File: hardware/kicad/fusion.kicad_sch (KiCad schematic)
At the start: 7 parts, among them J1 Battery, U1 MCP1603

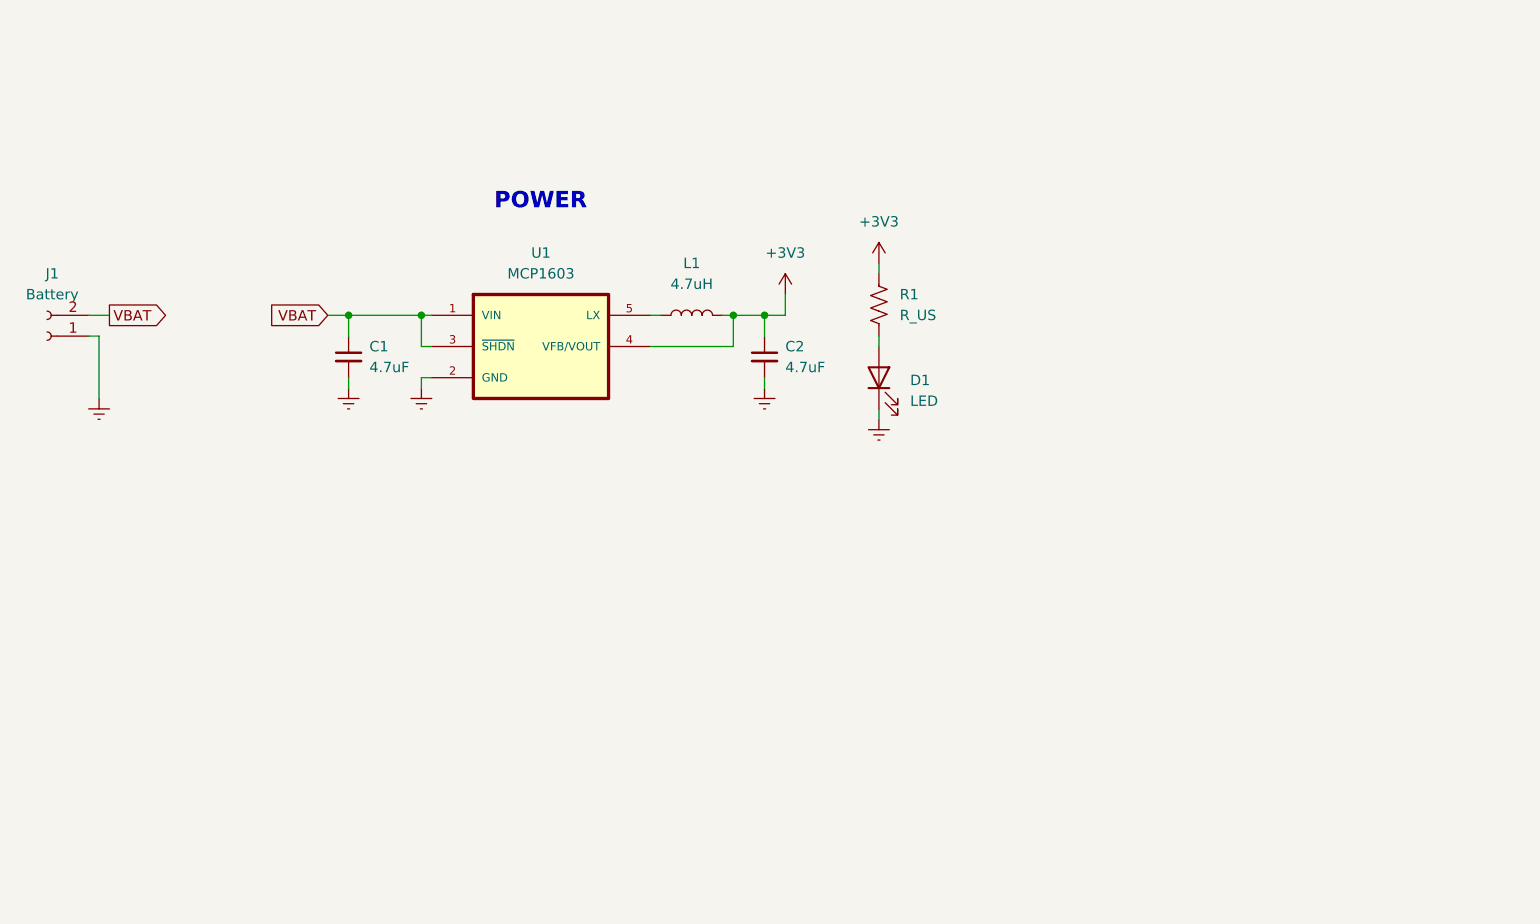
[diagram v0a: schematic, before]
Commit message: IMU SPI header
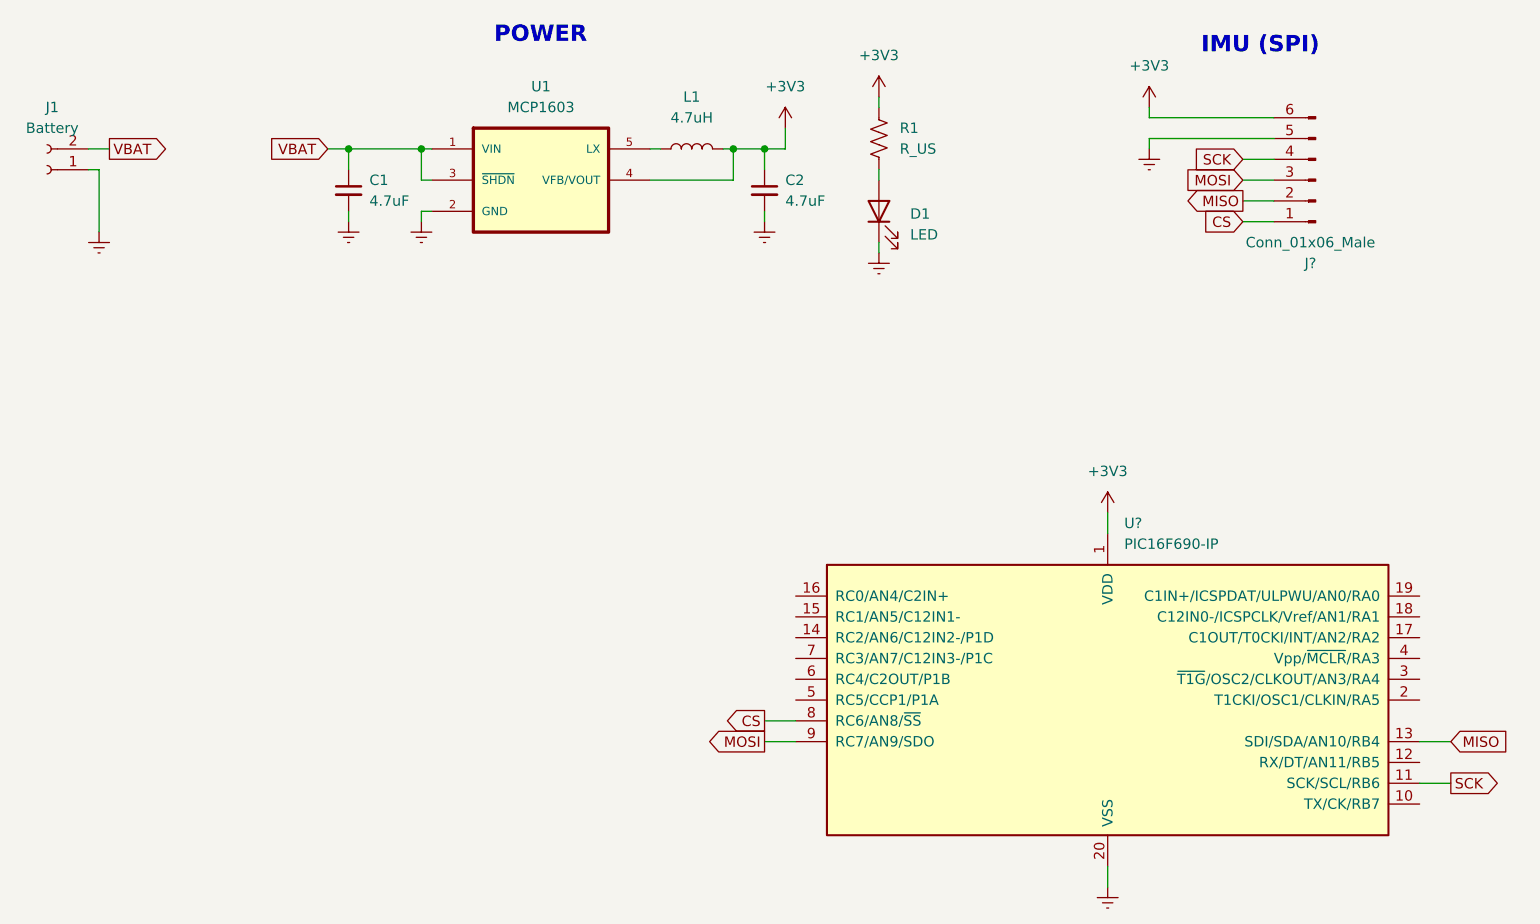
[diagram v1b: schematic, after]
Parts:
- added J?: Conn_01x06_Male, symbol Connector:Conn_01x06_Male
- added U?: PIC16F690-IP, symbol MCU_Microchip_PIC16:PIC16F690-IP
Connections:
- net +3V3: now also J?.6 (Pin_6), U?.1 (VDD)
- net GNDREF: now also J?.5 (Pin_5), U?.20 (VSS)
- new net CS: J?.1 (Pin_1), U?.8 (RC6/AN8/~{SS})
- new net MISO: J?.2 (Pin_2), U?.13 (SDI/SDA/AN10/RB4)
- new net MOSI: J?.3 (Pin_3), U?.9 (RC7/AN9/SDO)
- new net SCK: J?.4 (Pin_4), U?.11 (SCK/SCL/RB6)
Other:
- note added: "IMU (SPI)"
- moved on the sheet: C1, C2, D1, J1, L1, R1, U1
